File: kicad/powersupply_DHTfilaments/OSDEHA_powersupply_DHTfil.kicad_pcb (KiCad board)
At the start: 2 copper layers, 98.5 x 26 mm, 15 parts

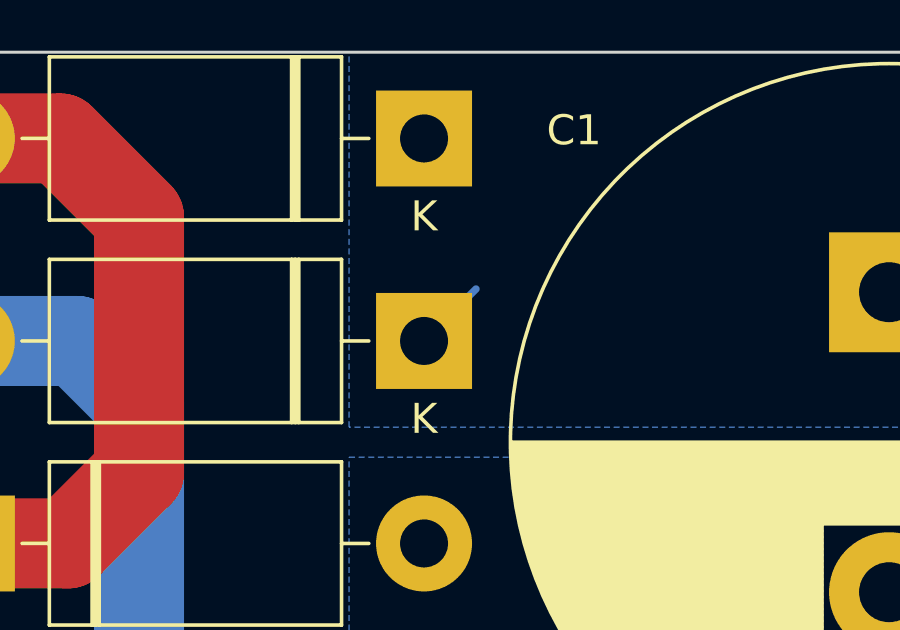
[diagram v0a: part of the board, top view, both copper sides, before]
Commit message: minor clean
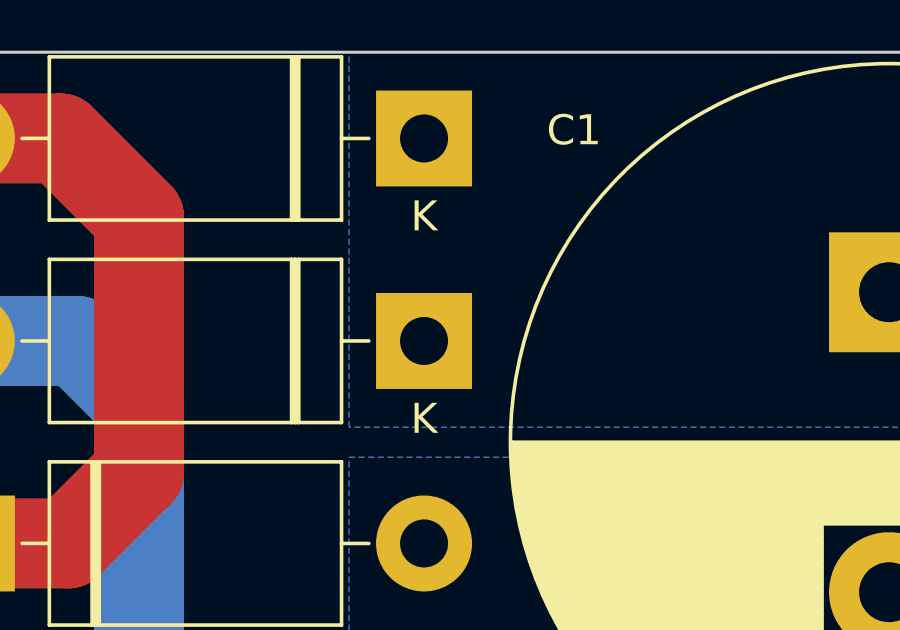
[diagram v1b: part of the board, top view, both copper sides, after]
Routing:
- net /R+: track 22.3 -> 19.9 mm
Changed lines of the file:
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@@
-	)
-	(segment
-		(start 100.73037 76.39463)
-		(end 99 78.125)
-		(width 0.25)
-		(layer "B.Cu")
-		(net 5)
 	)
 	(segment
